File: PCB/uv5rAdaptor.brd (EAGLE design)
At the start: 13.9 x 13.9 mm, 2 parts

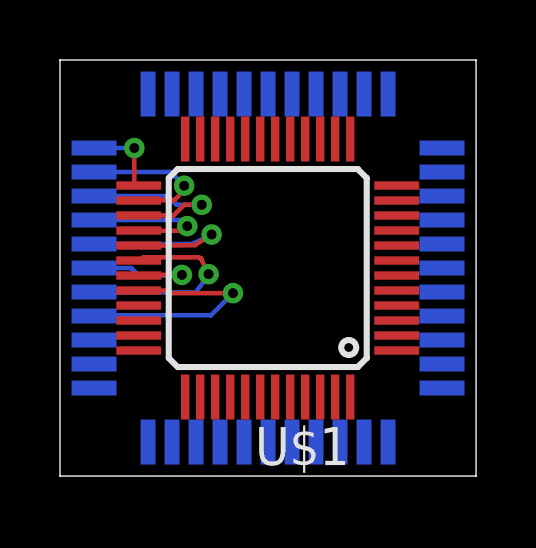
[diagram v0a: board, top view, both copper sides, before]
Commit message: More routing
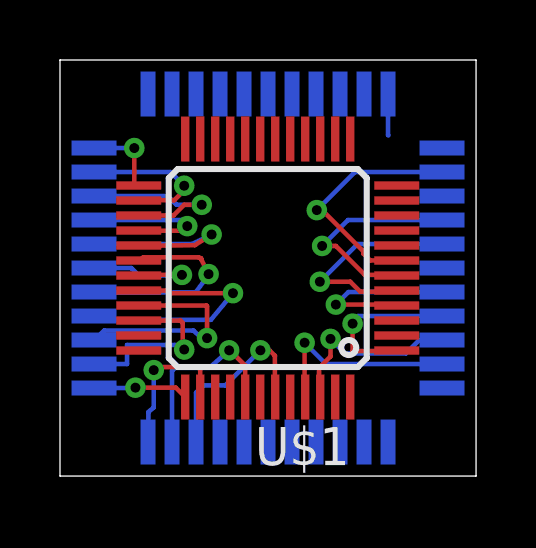
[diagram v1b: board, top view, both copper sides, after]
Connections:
- removed net N$50: U$1.45
- removed net NC1: U$1.38
- removed net NC11: U$1.46
- new net NC3: U$1.2
- new net NC4: U$1.3
- net LED_FL: now also U$1.38
- net SPK_AMP: now also U$1.46; no longer U$1.3
- net TX_PW: now also U$1.45; no longer U$1.2
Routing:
- net RESET: track 0.00 -> 8.11 mm, vias 0 -> 1
- net LCD_RS: track 0.00 -> 7.54 mm, vias 0 -> 1
- net OSC_IN: track 0.00 -> 7.31 mm, vias 0 -> 1
- net OSC_OUT: track 0.00 -> 7.25 mm, vias 0 -> 1
- net TX_PW: track 0.00 -> 6.69 mm, vias 0 -> 1
- net UHF/VHF: track 0.00 -> 6.33 mm, vias 0 -> 1
- net GREEN_LED: track 0.00 -> 6.32 mm, vias 0 -> 1
- net SPK_AMP: track 0.00 -> 6.21 mm, vias 0 -> 1
- net LCD_CE: track 0.00 -> 6.08 mm, vias 0 -> 1
- net VOX: track 0.00 -> 5.76 mm, vias 0 -> 1
- net LOW_BAT: track 0.00 -> 5.51 mm, vias 0 -> 1
- net LED_FL: track 0.00 -> 5.09 mm, vias 0 -> 1
- net RED_LED: track 0.00 -> 3.17 mm, vias 0 -> 1
- net SEN: track 0.00 -> 1.39 mm

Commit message: More traces
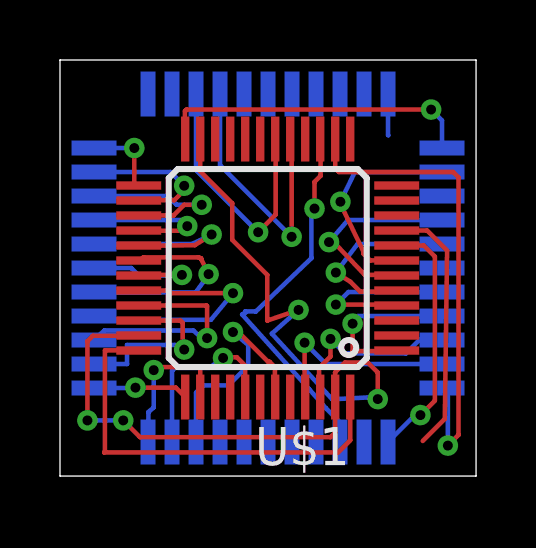
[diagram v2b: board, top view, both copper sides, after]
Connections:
- net KEY_C4: now also U$1.19; no longer U$1.20
- net RX_PW: now also U$1.20; no longer U$1.19
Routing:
- net VSS: track 0.00 -> 31.4 mm, vias 0 -> 4
- net VDD: track 0.00 -> 24.9 mm, vias 0 -> 1
- net TX_BIAS: track 0.00 -> 16.3 mm, vias 0 -> 1
- net TONE: track 0.00 -> 12.7 mm, vias 0 -> 1
- net GPIO0: track 0.00 -> 9.03 mm, vias 0 -> 1
- net CLK_FM: track 0.00 -> 8.82 mm, vias 0 -> 1
- net AVDD: track 0.00 -> 8.61 mm
- net AVSS: track 0.00 -> 8.36 mm, vias 0 -> 1
- net GREEN_LED: track 6.32 -> 7.99 mm
- net OSC_IN: track 7.31 -> 6.28 mm
- net RESET: track 8.11 -> 7.11 mm
